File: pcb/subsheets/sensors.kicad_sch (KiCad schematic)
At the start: 7 parts, among them U2 Barometer-KP212K1409XTMA1, U3 Thermometer-LM335D

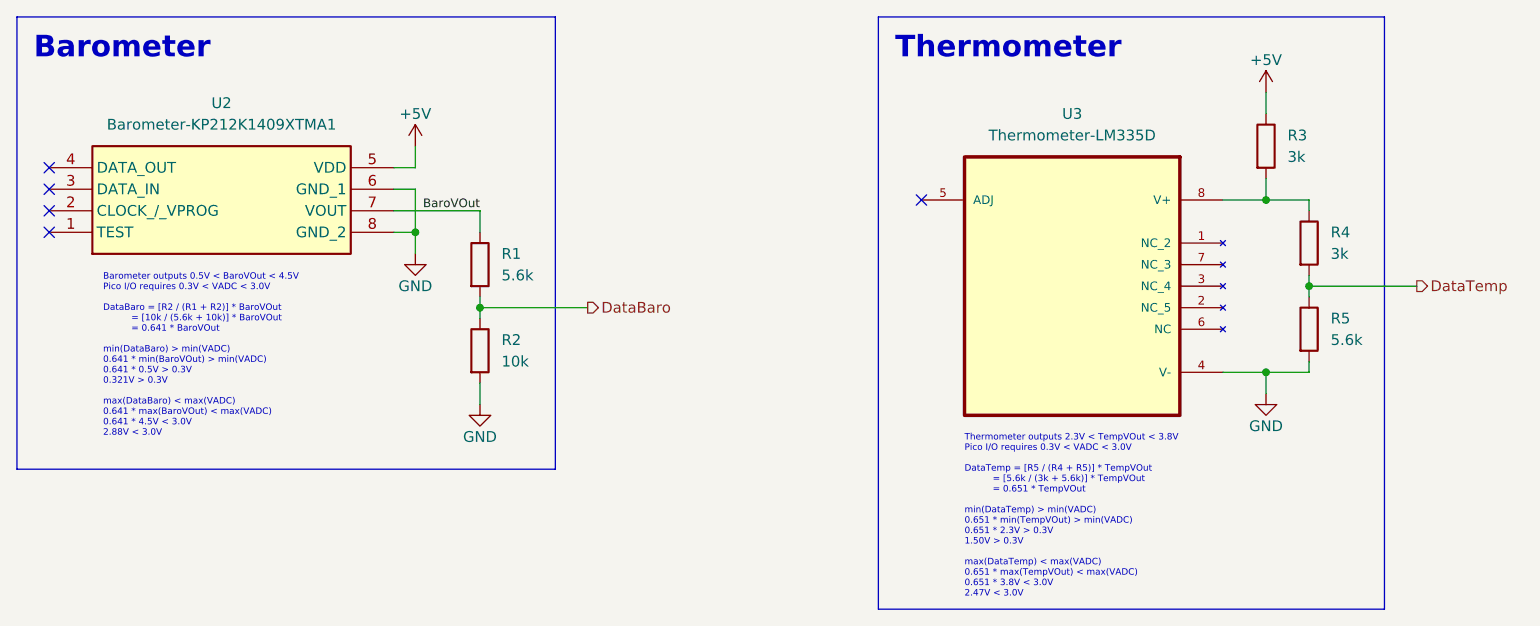
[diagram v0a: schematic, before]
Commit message: fixed everything (ERC is no longer mad)
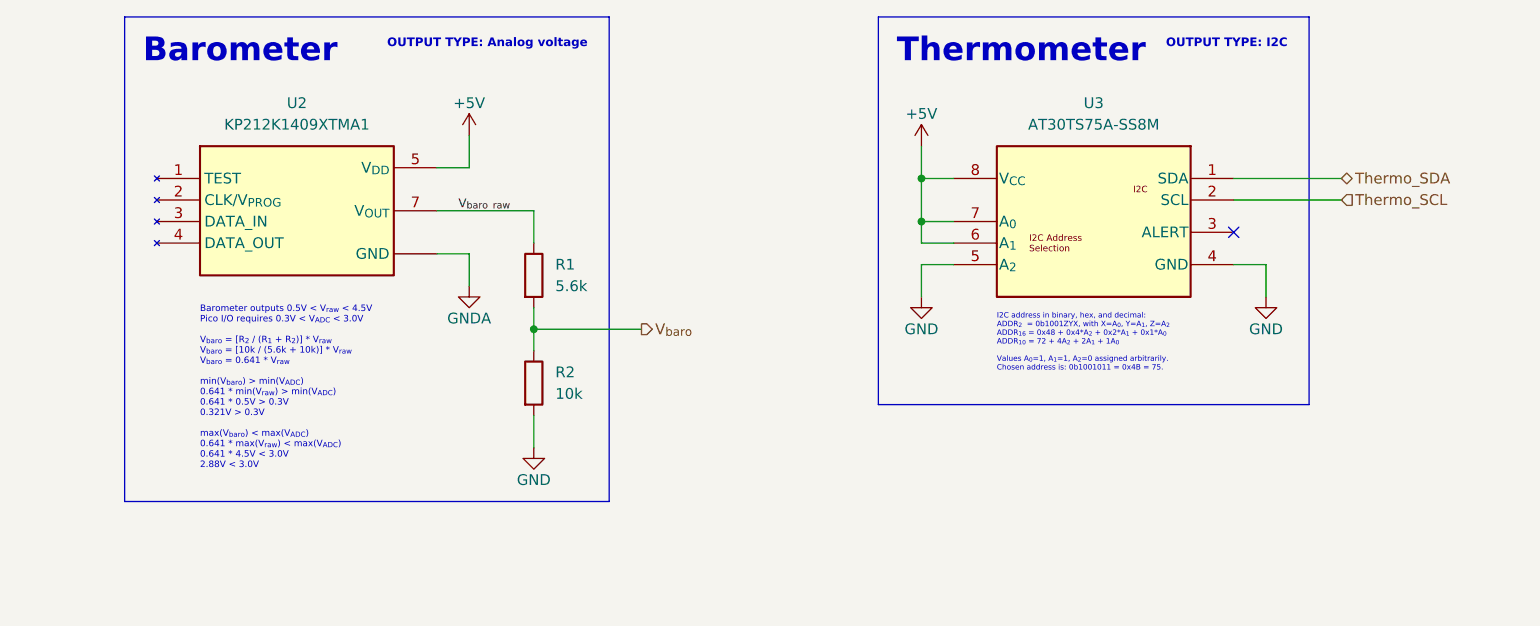
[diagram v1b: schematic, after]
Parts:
- removed R3, R4: 3k, symbol Device:R
- removed R5: 5.6k, symbol Device:R
- removed U3: Thermometer-LM335D, BeltFootprints:Thermometer-LM335D, symbol Thermometer-LM335D:Thermometer-LM335D
- added U3: AT30TS75A-SS8M, BeltFootprints:Thermometer-AT30TS75A-SS8M, symbol Thermometer-AT30TS75A-SS8M:Thermometer-AT30TS75A-SS8M
- U2: value Barometer-KP212K1409XTMA1 -> KP212K1409XTMA1
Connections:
- net +5V: now also U3.6 (A_{1}), U3.7 (A_{0}), U3.8 (V_{CC})
- net GND: now also U3.4 (GND), U3.5 (A_{2}); no longer U2.6 (GND_1), U2.8 (GND_2)
- net BaroVOut renamed V_{baro_raw}
- net DataBaro renamed V_{baro}
- new net GNDA: U2.6 (GND), U2.8 (GND)
- new net Thermo_SCL: U3.2 (SCL)
- new net Thermo_SDA: U3.1 (SDA)
- no-connect marks 5 -> 1
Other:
- note added: "Barometer outputs 0.5V < V_{raw} < 4.5V Pico I/O requires 0.3V < V_{ADC} < 3.0V V_{baro} = [R_{2} / (R_{1} + R_{2})] * V_{raw} V_{baro} = [10k / (5.6k + 10k)] * V_{raw} V_{baro} = 0.641 * V_{raw} min(V_{baro}) > min(V_{ADC}) 0.641 * min(V_{raw}) > min(V_{ADC}) 0.641 * 0.5V > 0.3V 0.321V > 0.3V max(V_{baro}) < max(V_{ADC}) 0.641 * max(V_{raw}) < max(V_{ADC}) 0.641 * 4.5V < 3.0V 2.88V < 3.0V"
- note added: "I2C address in binary, hex, and decimal: ADDR_{2} = 0b1001ZYX, with X=A_{0}, Y=A_{1}, Z=A_{2} ADDR_{16} = 0x48 + 0x4*A_{2} + 0x2*A_{1} + 0x1*A_{0} ADDR_{10} = 72 + 4A_{2} + 2A_{1} + 1A_{0} Values A_{0}=1, A_{1}=1, A_{2}=0 assigned arbitrarily. Chosen address is: 0b1001011 = 0x4B = 75."
- note added: "OUTPUT TYPE: Analog voltage"
- note added: "OUTPUT TYPE: I2C"
- note removed: "Barometer outputs 0.5V < BaroVOut < 4.5V Pico I/O requires 0.3V < VADC < 3.0V DataBaro = [R2 / (R1 + R2)] * BaroVOut = [10k / (5.6k + 10k)] * BaroVOut = 0.641 * BaroVOut min(DataBaro) > min(VADC) 0.641 * min(BaroVOut) > min(VADC) 0.641 * 0.5V > 0.3V 0.321V > 0.3V max(DataBaro) < max(VADC) 0.641 * max(BaroVOut) < max(VADC) 0.641 * 4.5V < 3.0V 2.88V < 3.0V"
- note removed: "Thermometer outputs 2.3V < TempVOut < 3.8V Pico I/O requires 0.3V < VADC < 3.0V DataTemp = [R5 / (R4 + R5)] * TempVOut = [5.6k / (3k + 5.6k)] * TempVOut = 0.651 * TempVOut min(DataTemp) > min(VADC) 0.651 * min(TempVOut) > min(VADC) 0.651 * 2.3V > 0.3V 1.50V > 0.3V max(DataTemp) < max(VADC) 0.651 * max(TempVOut) < max(VADC) 0.651 * 3.8V < 3.0V 2.47V < 3.0V"
